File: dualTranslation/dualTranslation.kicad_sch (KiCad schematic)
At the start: 53 parts, among them IC1 LSF0108PWR, IC2 LSF0108PWR, J1 L_dual, J2 R_dual, J6 MISC, Q1 MMBT3904, Q2 MMBT3904

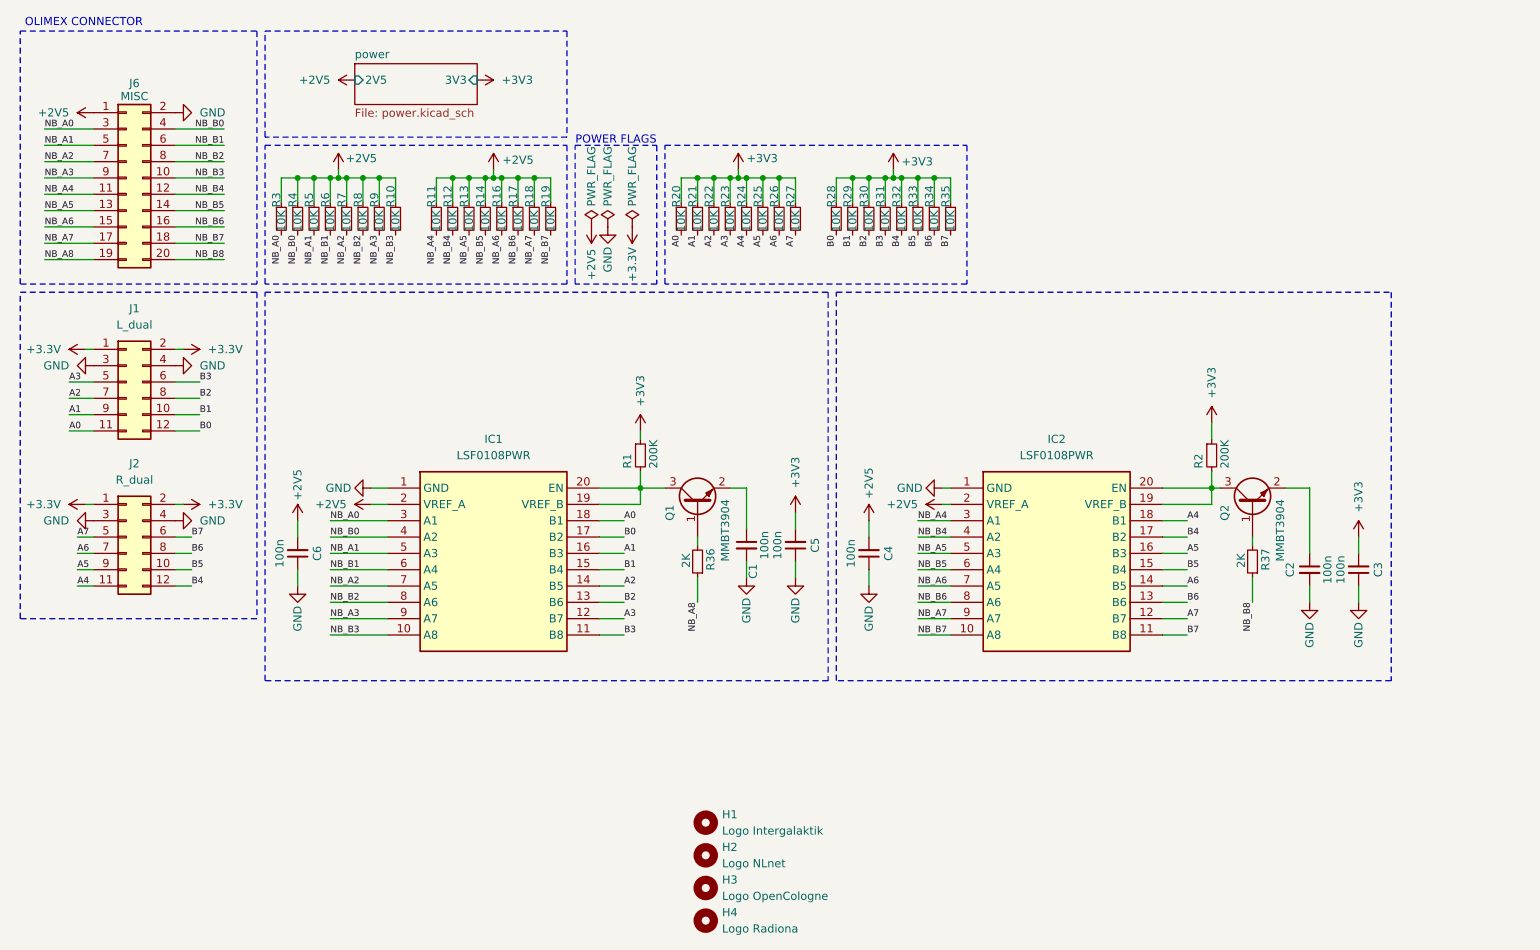
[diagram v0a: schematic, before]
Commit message: Routing
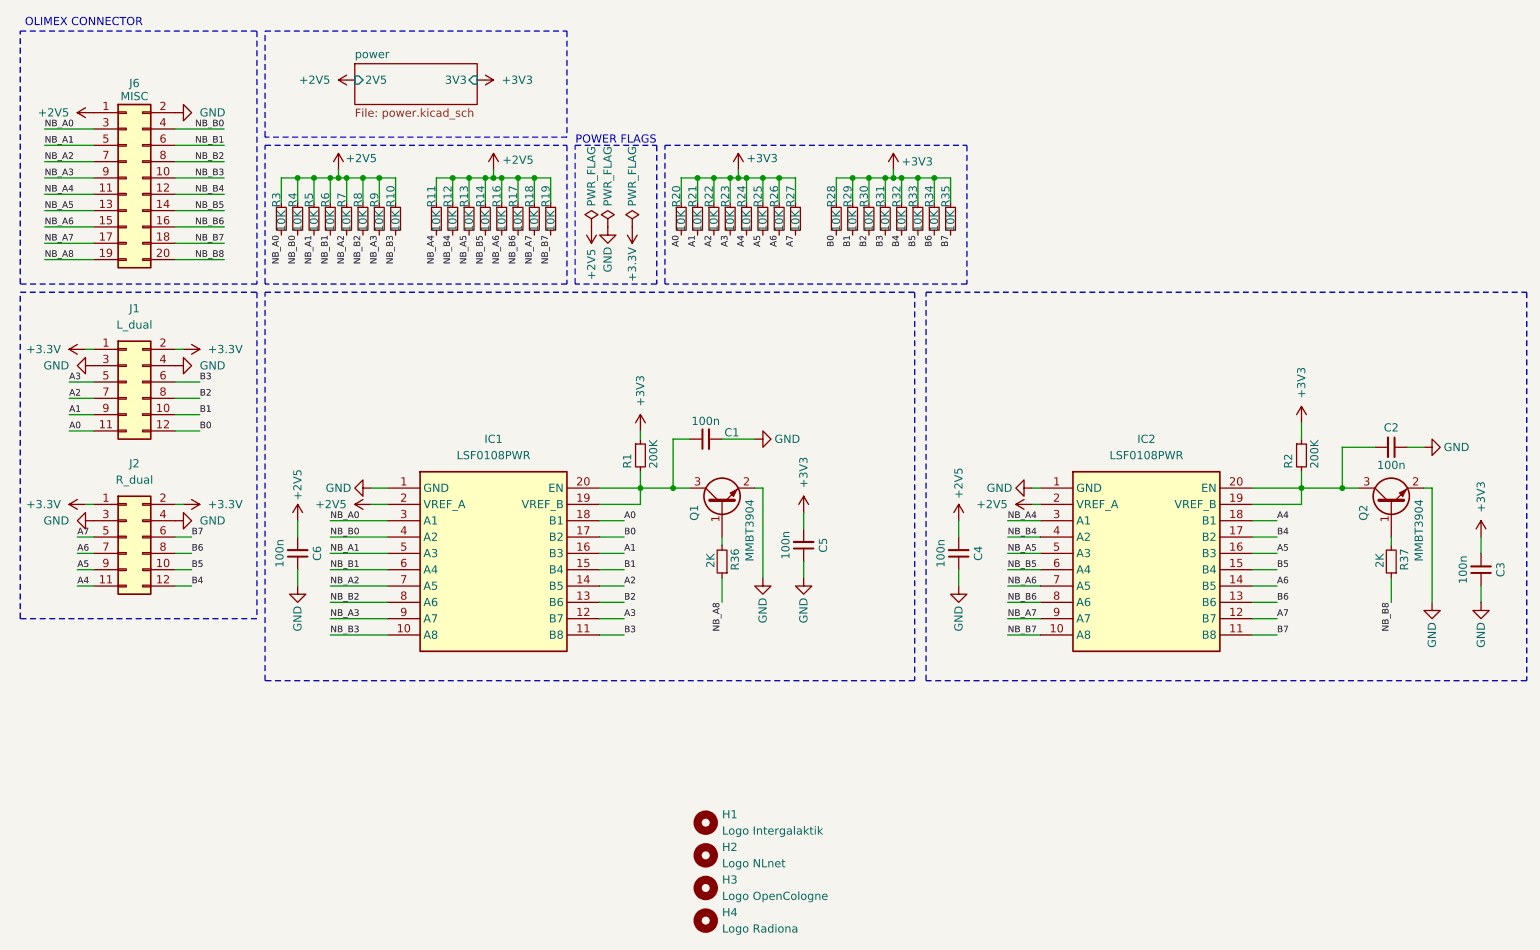
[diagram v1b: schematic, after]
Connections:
- net GND: now also C2.1, Q1.2 (E), Q2.2 (E); no longer C2.2
- net at IC1.19 (VREF_B), IC1.20 (EN), Q1.3 (C)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: now also C1.1
- net at IC2.19 (VREF_B), IC2.20 (EN), Q2.3 (C)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: now also C2.2
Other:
- moved on the sheet: C1, C2, C3, C4, C5, IC2, Q1, Q2, R2, R36, R37
